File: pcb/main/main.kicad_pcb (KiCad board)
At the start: 2 copper layers, 44.5 x 74.9 mm, 96 parts, among them J1 USB_C_Receptacle_USB2.0, J10 COL4, J11 COL6, J12 OLED, J13 Conn_01x05_Female, J14 OLED, J2 RJ45, J3 RJ45, J4 Pad, J5 Thumb, J6 COL1, J7 COL5, J8 COL2, J9 COL3, SW1 SW_SPDT, SW2 SW_SPDT, SW3 RESET, U1 STM32F401RETx, U2 NATLINEAR XT1861B332MR-G, U3 PCA9306DC1, U4 HT7727, Y1 Crystal_8MHz, Y2 Crystal_32.768MHz

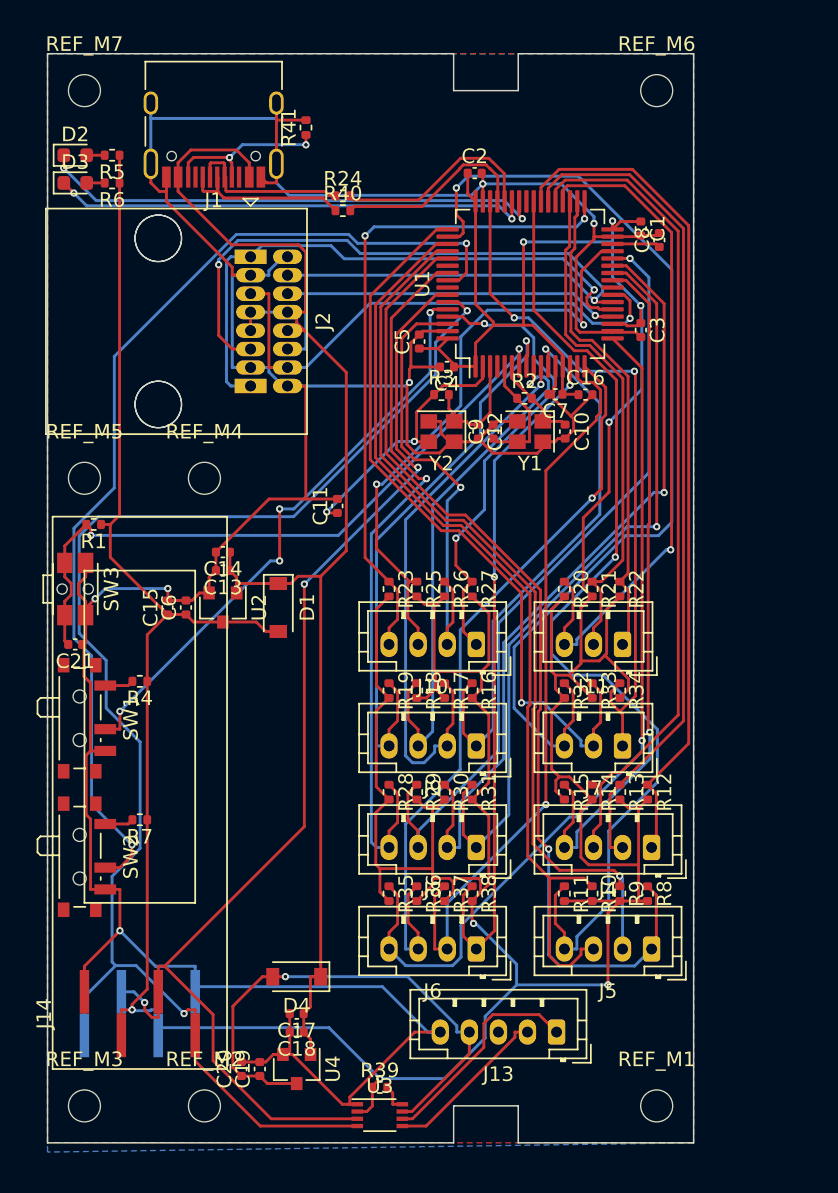
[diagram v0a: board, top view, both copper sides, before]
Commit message: redesign pcb
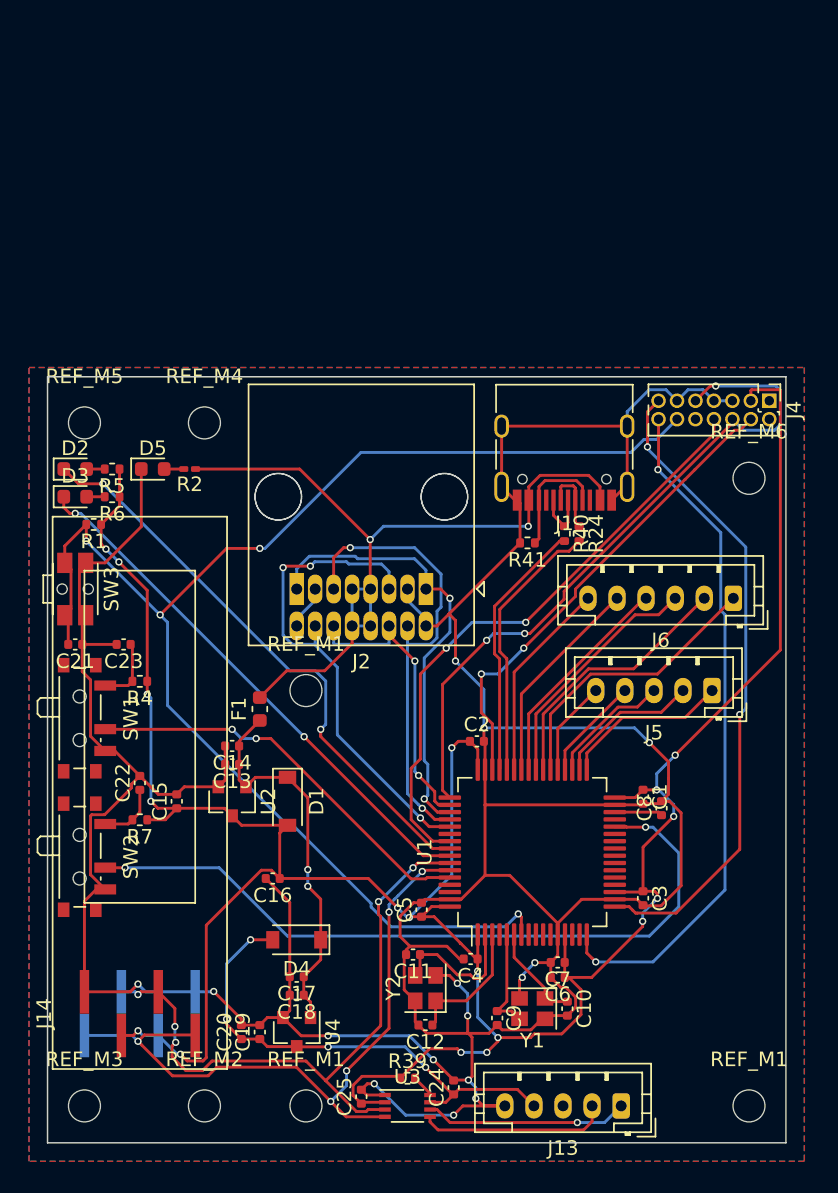
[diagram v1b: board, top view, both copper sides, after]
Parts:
- removed J10: COL4, Connector_JST:JST_PH_B4B-PH-K_1x04_P2.00mm_Vertical
- removed J11: COL6, Connector_JST:JST_PH_B3B-PH-K_1x03_P2.00mm_Vertical
- removed J7: COL5, Connector_JST:JST_PH_B3B-PH-K_1x03_P2.00mm_Vertical
- removed J8: COL2, Connector_JST:JST_PH_B4B-PH-K_1x04_P2.00mm_Vertical
- removed J9: COL3, Connector_JST:JST_PH_B4B-PH-K_1x04_P2.00mm_Vertical
- removed R10, R11, R12, R13, R14, R15, R16, R17, R18, R19, R20, R21, R22, R23, R25, R26, R27, R28, R29, R30, R31, R32, R33, R34, R35, R36, R37, R38, R8, R9: 10k, Resistor_SMD:R_0402_1005Metric
- removed R3: 10M, Resistor_SMD:R_0402_1005Metric
- removed REF_M7: MountingHole_2.2mm_M2, MountingHole:MountingHole_2.2mm_M2
- added C22: 0.1uF, Capacitor_SMD:C_0402_1005Metric, F.Cu at (6.35, -24.8)
- added C23: 0.1uF, Capacitor_SMD:C_0402_1005Metric, F.Cu at (5.24, -34.3)
- added C24: 0.1uF, Capacitor_SMD:C_0402_1005Metric, F.Cu at (27.9, -3.81)
- added C25: 0.1uF, Capacitor_SMD:C_0402_1005Metric, F.Cu at (21.6, -3.17)
- added D5: LED_USB, LED_SMD:LED_0603_1608Metric, F.Cu at (7.24, -46.4)
- added F1: Polyfuse, Fuse:Fuse_0603_1608Metric, F.Cu at (14.6, -29.8)
- added REF_M1: MountingHole_2.2mm_M2, MountingHole:MountingHole_2.2mm_M2, F.Cu at (17.8, -31.1)
- added REF_M1: MountingHole_2.2mm_M2, MountingHole:MountingHole_2.2mm_M2, F.Cu at (17.8, -2.54)
- J13: value Conn_01x05_Female -> trackball
- J4: value Pad -> STLink; footprint Connector_JST:JST_PH_B4B-PH-K_1x04_P2.00mm_Vertical -> Connector_PinHeader_1.27mm:PinHeader_2x07_P1.27mm_Vertical
- J5: value Thumb -> ROW; footprint Connector_JST:JST_PH_B4B-PH-K_1x04_P2.00mm_Vertical -> Connector_JST:JST_PH_B5B-PH-K_1x05_P2.00mm_Vertical
- J6: value COL1 -> COL; footprint Connector_JST:JST_PH_B4B-PH-K_1x04_P2.00mm_Vertical -> Connector_JST:JST_PH_B6B-PH-K_1x06_P2.00mm_Vertical
- R2: value 10M -> R; footprint Resistor_SMD:R_0402_1005Metric -> Resistor_SMD:R_0201_0603Metric_Pad0.64x0.40mm_HandSolder
- moved C12 41.0 mm to (26.0, -8.10), turned to 180 degrees
- moved C4 40.8 mm to (29.1, -12.6)
- moved C9 40.3 mm to (30.9, -8.59), turned to 270 degrees
- moved C10 39.7 mm to (35.8, -9.23)
- moved Y1 39.7 mm to (33.4, -9.23)
- moved C16 39.6 mm to (15.5, -18.2), turned to 180 degrees
- moved C1 39.1 mm to (41.0, -23.8)
- moved C3 39.1 mm to (41.0, -16.8)
- moved C5 39.1 mm to (25.7, -16.0)
- moved C7 39.1 mm to (35.1, -12.4)
- moved C8 39.1 mm to (42.2, -23.0)
- moved C2 39.1 mm to (29.5, -27.6)
- moved U1 39.1 mm to (33.4, -20.0)
- moved Y2 38.3 mm to (26.0, -10.6), turned to 90 degrees
- moved C6 36.1 mm to (35.1, -11.4), turned to 180 degrees
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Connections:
- C13 pad 1: VBUS -> Net-(C13-Pad1)
- C14 pad 1: VBUS -> Net-(C13-Pad1)
- C17 pad 1: VBUS -> Net-(C13-Pad1)
- C18 pad 1: VBUS -> Net-(C13-Pad1)
- C21 pad 2: Net-(C21-Pad2) -> /NRST
- D1 pad 1: VBUS -> Net-(C13-Pad1)
- D4 pad 1: VBUS -> Net-(C13-Pad1)
- J4 pad 1: Net-(J4-Pad1) -> (no net)
- J4 pad 2: Net-(J4-Pad2) -> (no net)
- J4 pad 3: Net-(J4-Pad3) -> +3V3
- J4 pad 4: Net-(J4-Pad4) -> /SWDIO
- J5 pad 1: Net-(J5-Pad1) -> /ROW1
- J5 pad 2: Net-(J5-Pad2) -> /ROW2
- J5 pad 3: Net-(J5-Pad3) -> /ROW3
- J5 pad 4: Net-(J5-Pad4) -> /ROW4
- J6 pad 1: Net-(J6-Pad1) -> /COL1
- J6 pad 2: Net-(J6-Pad2) -> /COL2
- J6 pad 3: Net-(J6-Pad3) -> /COL3
- J6 pad 4: Net-(J6-Pad4) -> /COL4
- R1 pad 2: Net-(C21-Pad2) -> /NRST
- R2 pad 1: /XTAL1A -> VBUS
- R2 pad 2: /XTAL1B -> Net-(D5-Pad2)
- SW2 pad 2: /CONFIG -> /BOOT1
- SW3 pad 2: Net-(C21-Pad2) -> /NRST
- U1 pad 10: Net-(J9-Pad2) -> (no net)
- U1 pad 11: Net-(J9-Pad1) -> (no net)
- U1 pad 14: Net-(J6-Pad1) -> (no net)
- U1 pad 15: Net-(J6-Pad2) -> (no net)
- U1 pad 16: Net-(J6-Pad3) -> /TX
- U1 pad 17: Net-(J6-Pad4) -> /RX
- U1 pad 20: /SS -> (no net)
- U1 pad 21: /SCLK -> (no net)
- U1 pad 22: /MISO -> (no net)
- U1 pad 23: /MOSI -> (no net)
- U1 pad 25: Net-(J4-Pad4) -> (no net)
- U1 pad 26: Net-(J8-Pad1) -> (no net)
- U1 pad 27: Net-(J8-Pad2) -> (no net)
- U1 pad 28: Net-(J8-Pad3) -> /BOOT1
- U1 pad 29: Net-(J10-Pad3) -> (no net)
- U1 pad 33: Net-(J10-Pad4) -> /ROW1
- U1 pad 34: Net-(J11-Pad1) -> /ROW2
- U1 pad 35: Net-(J11-Pad2) -> /ROW3
- U1 pad 36: Net-(J11-Pad3) -> /ROW4
- U1 pad 37: Net-(J4-Pad3) -> /ROW5
- U1 pad 38: Net-(J4-Pad2) -> /COL1
- U1 pad 39: Net-(J4-Pad1) -> /COL2
- U1 pad 40: Net-(J5-Pad4) -> /COL3
- U1 pad 41: (no net) -> /COL4
- U1 pad 42: /LED_ERROR -> /COL5
- U1 pad 43: /LED_STATUS -> /COL6
- U1 pad 46: Net-(J7-Pad1) -> /SWDIO
- U1 pad 49: Net-(J7-Pad2) -> /SWCLK
- U1 pad 50: Net-(J7-Pad3) -> /SS
- U1 pad 51: Net-(J5-Pad3) -> /SCLK
- U1 pad 52: Net-(J5-Pad2) -> /MISO
- U1 pad 53: Net-(J5-Pad1) -> /MOSI
- U1 pad 55: Net-(J8-Pad4) -> /SWO
- U1 pad 56: /CONFIG -> /LED_ERROR
- U1 pad 57: (no net) -> /LED_STATUS
- U1 pad 61: Net-(J10-Pad1) -> (no net)
- U1 pad 62: Net-(J10-Pad2) -> (no net)
- U1 pad 7: Net-(C21-Pad2) -> /NRST
- U1 pad 8: Net-(J9-Pad4) -> (no net)
- U1 pad 9: Net-(J9-Pad3) -> (no net)
- U2 pad 1: VBUS -> Net-(C13-Pad1)
- U4 pad 1: VBUS -> Net-(C13-Pad1)
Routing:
- net +3V3: track 345.4 -> 191.7 mm, vias 8 -> 18
- net /NRST: track 0.00 -> 97.7 mm, vias 0 -> 4
- net /CONFIG: track 70.8 -> 0.00 mm, vias 2 -> 0
- net Net-(J5-Pad4): track 68.4 -> 0.00 mm, vias 1 -> 0
- net Net-(J5-Pad1): track 68.2 -> 0.00 mm, vias 1 -> 0
- net Net-(J7-Pad3): track 67.6 -> 0.00 mm, vias 1 -> 0
- net Net-(J5-Pad3): track 64.5 -> 0.00 mm
- net Net-(J5-Pad2): track 61.0 -> 0.00 mm, vias 1 -> 0
- net Net-(J6-Pad4): track 59.3 -> 0.00 mm, vias 1 -> 0
- net Net-(J4-Pad2): track 57.7 -> 0.00 mm
- net Net-(J4-Pad1): track 57.6 -> 0.00 mm
- net Net-(J4-Pad3): track 56.7 -> 0.00 mm
- net Net-(J8-Pad2): track 53.9 -> 0.00 mm, vias 1 -> 0
- net Net-(J8-Pad3): track 53.7 -> 0.00 mm, vias 1 -> 0
- net Net-(J8-Pad1): track 52.6 -> 0.00 mm, vias 1 -> 0
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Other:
- board size 44.5 x 74.9 mm -> 50.8 x 52.7 mm

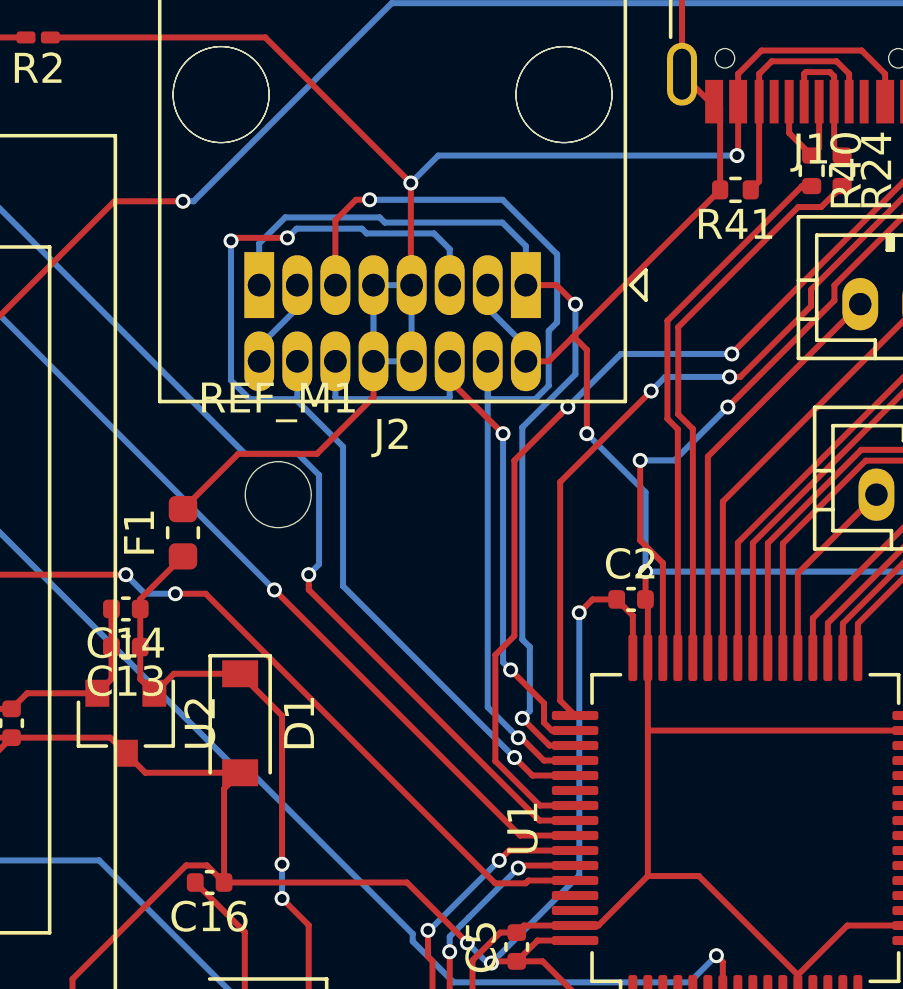
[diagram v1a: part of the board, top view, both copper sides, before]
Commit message: finish
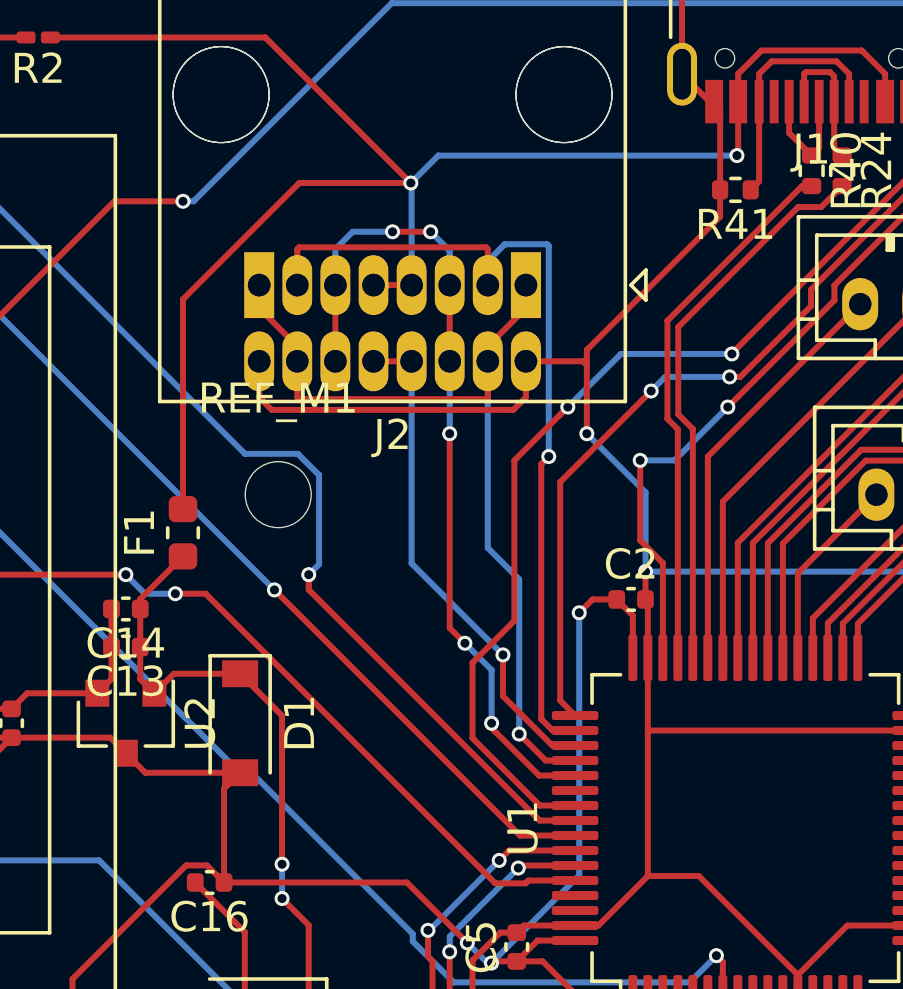
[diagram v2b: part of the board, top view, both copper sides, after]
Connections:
- J2 pad 1: /SCLK -> /MISO
- J2 pad 4: VBUS -> /SCLK
- J2 pad 6: /SS -> /MOSI
- J2 pad 7: GND -> /SS
- J3 pad 1: /SCLK -> /MISO
- J3 pad 2: /MOSI -> /MISO
- J3 pad 3: /MISO -> /MOSI
- J3 pad 4: VBUS -> /SCLK
- J3 pad 6: /SS -> /MOSI
- J3 pad 7: GND -> /SS
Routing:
- net /SCLK: track 31.1 -> 16.8 mm, vias 2 -> 1
- net /SS: track 20.8 -> 29.0 mm, vias 2 -> 1
- net /MOSI: track 34.5 -> 28.0 mm, vias 3 -> 5
- net GND: track 282.7 -> 288.0 mm
- net /MISO: track 33.7 -> 30.0 mm, vias 2 -> 1
- net VBUS: track 54.6 -> 55.4 mm
- net /SWO: track 41.6 -> 42.2 mm
